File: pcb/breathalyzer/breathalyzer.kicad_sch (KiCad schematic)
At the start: 25 parts, among them J1 Conn_01x07_Pin, Q1 Q_PMOS, SW1 PTS636SK43SMTR, SW2 430162085826, U1 STM32F030K6Tx, U2 TLV73325PDBV, U4 TLV61070ADBV, U5 AY0438X-L

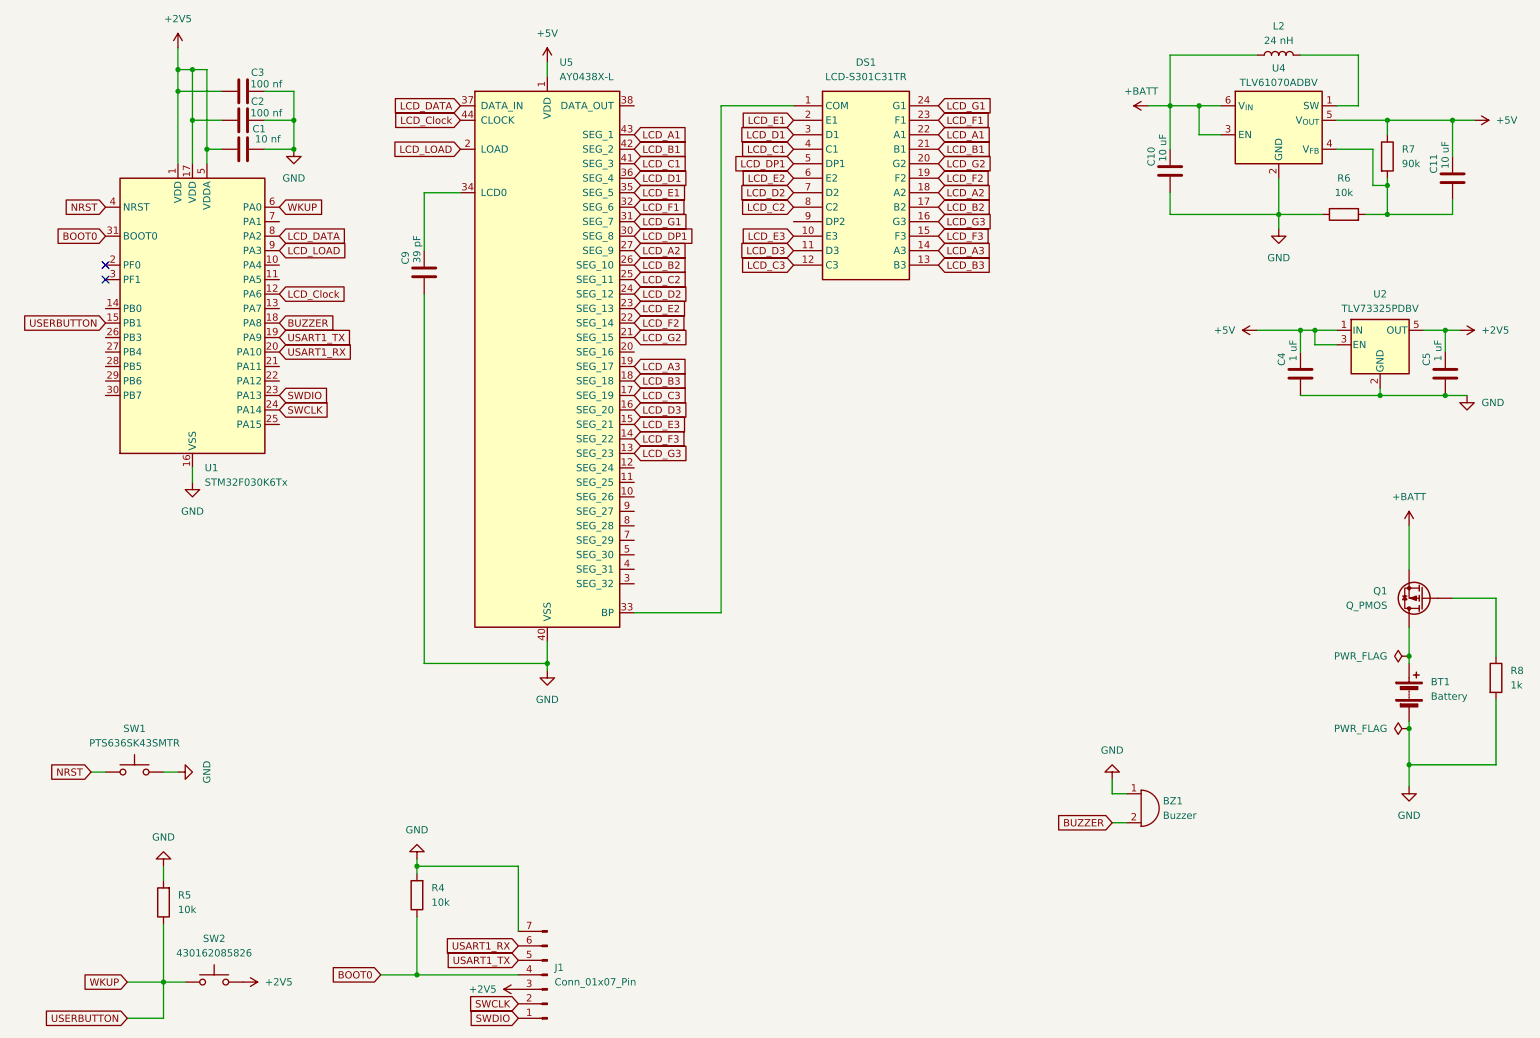
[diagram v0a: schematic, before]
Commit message: sensor connector
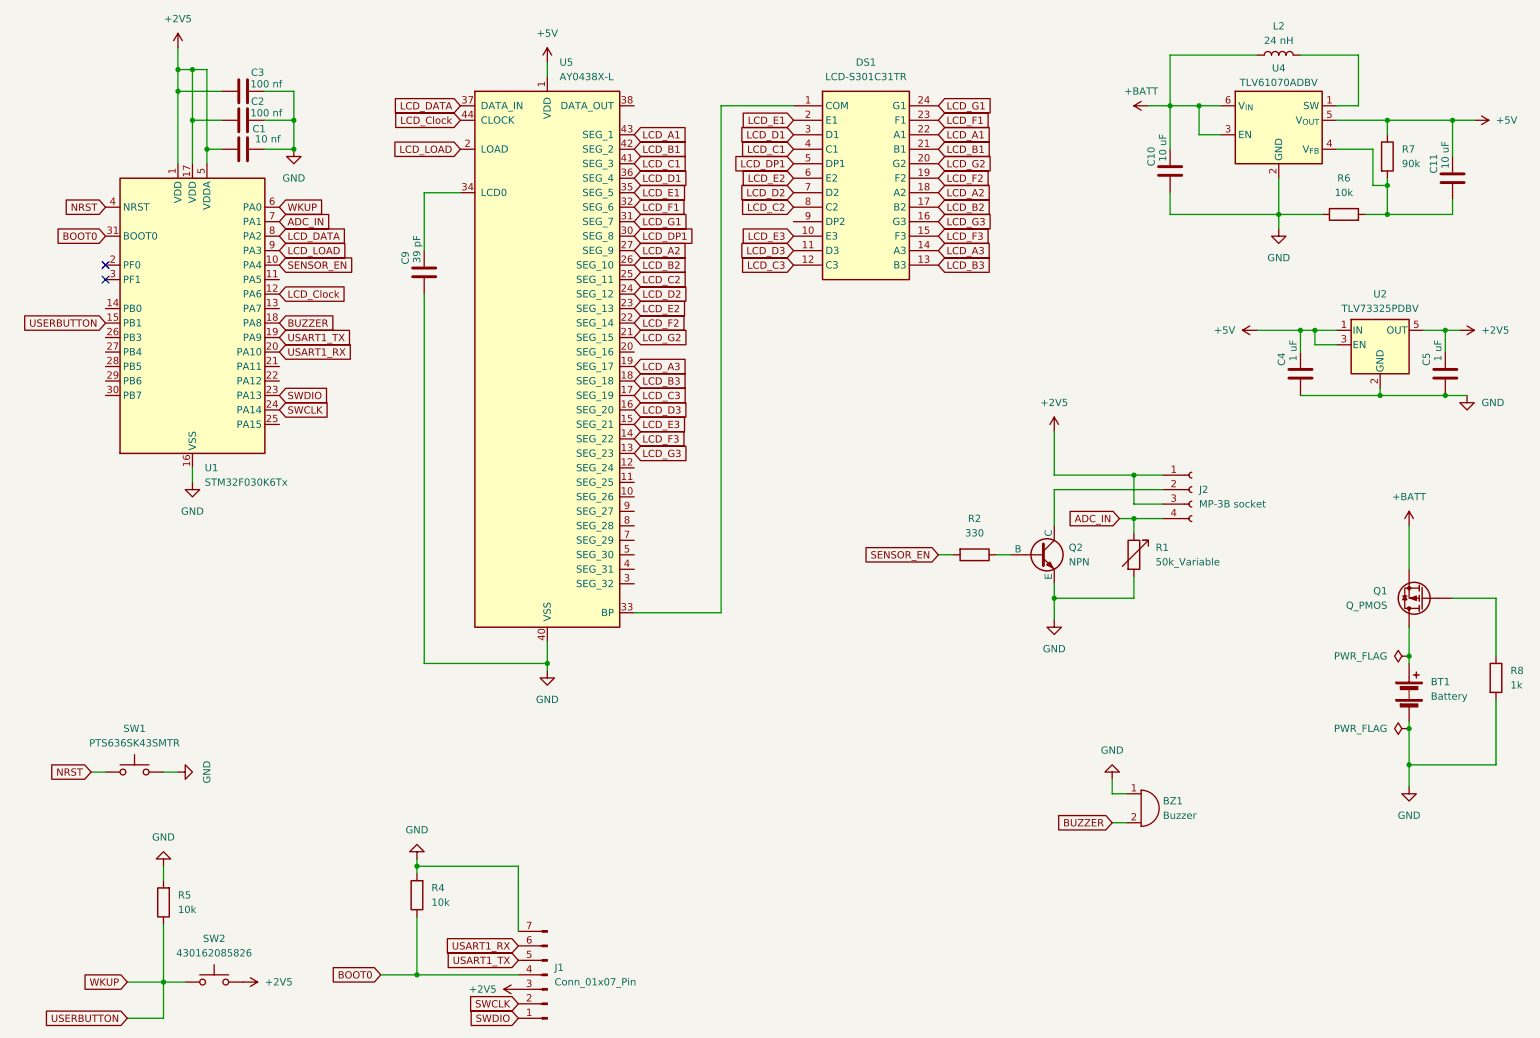
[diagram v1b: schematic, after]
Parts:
- added J2: MP-3B socket, breathalyzer:25SHB04TS, symbol Connector:Conn_01x04_Socket
- added Q2: NPN, Package_TO_SOT_SMD:SOT-23-3, symbol Simulation_SPICE:NPN
- added R1: 50k_Variable, Potentiometer_THT:Potentiometer_ACP_CA9-H5_Horizontal, symbol Device:R_Variable
- added R2: 330, Resistor_SMD:R_0805_2012Metric, symbol Device:R
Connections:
- net +2V5: now also J2.1 (Pin_1), J2.3 (Pin_3)
- net GND: now also Q2.3 (E), R1.2
- net SENSOR_EN: now reaches U1.10 (PA4)
- net SENSOR_EN: now also R2.2
- net ADC_IN: now reaches U1.7 (PA1)
- net ADC_IN: now also J2.4 (Pin_4), R1.1
- new net: J2.2 (Pin_2), Q2.1 (C)
- new net: Q2.2 (B), R2.1
